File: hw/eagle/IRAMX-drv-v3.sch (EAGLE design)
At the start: 59 parts, among them IC1 IRAMTOP, IC2 STM32F103R6T, IC3 78L05SMD, IC4 78L05SMD

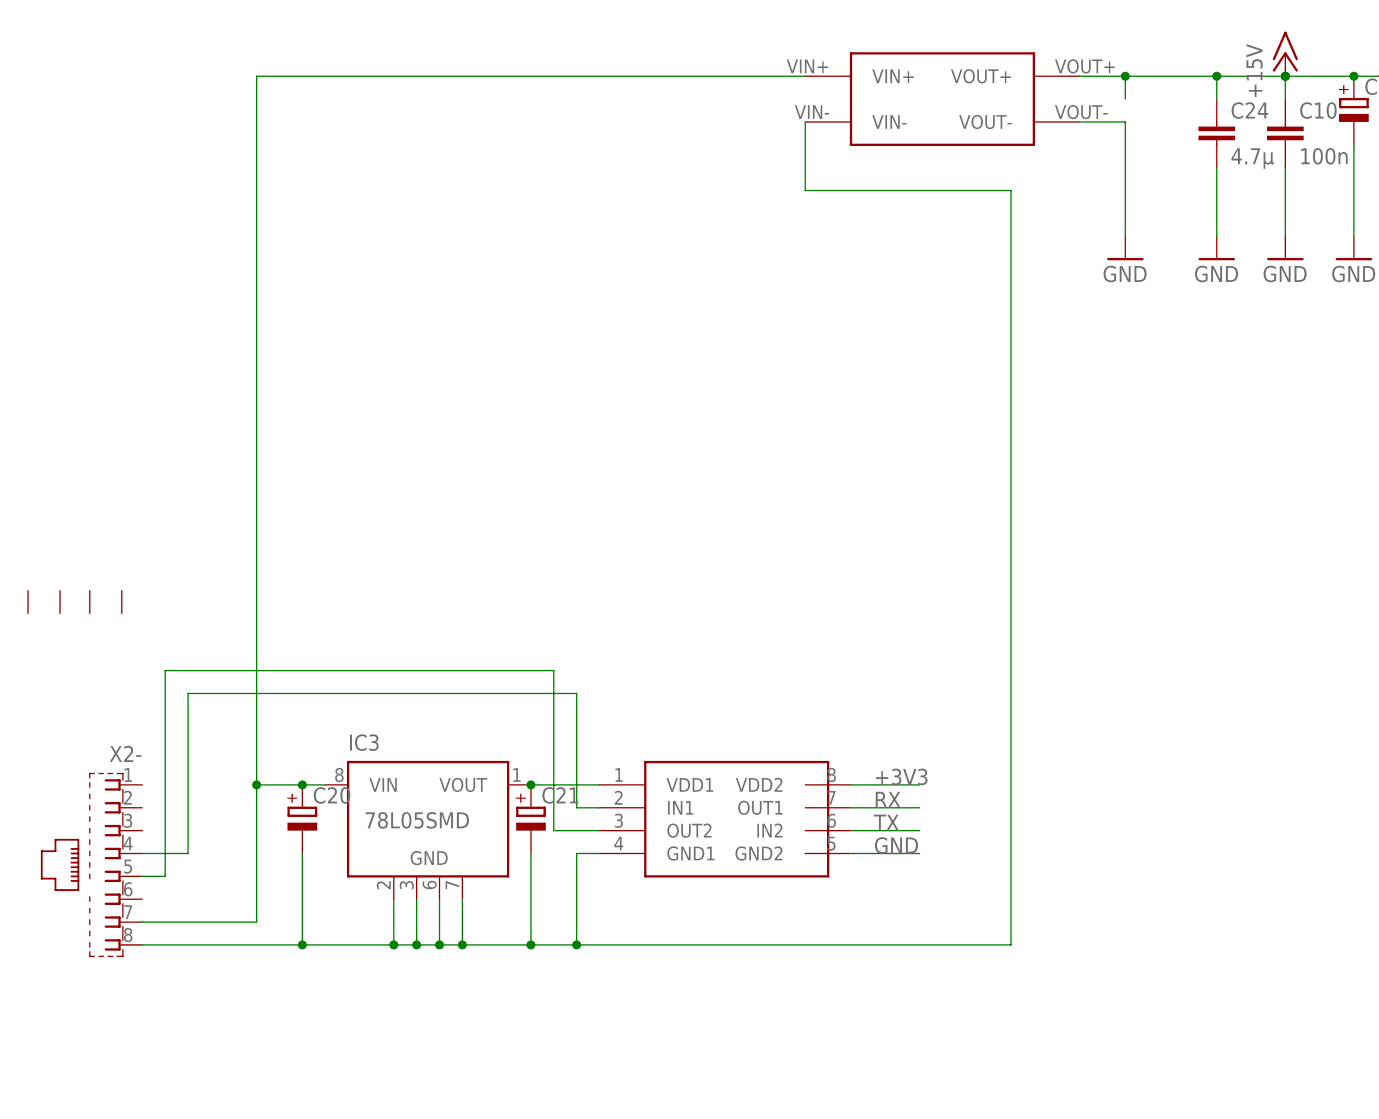
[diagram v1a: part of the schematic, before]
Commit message: iramx v3
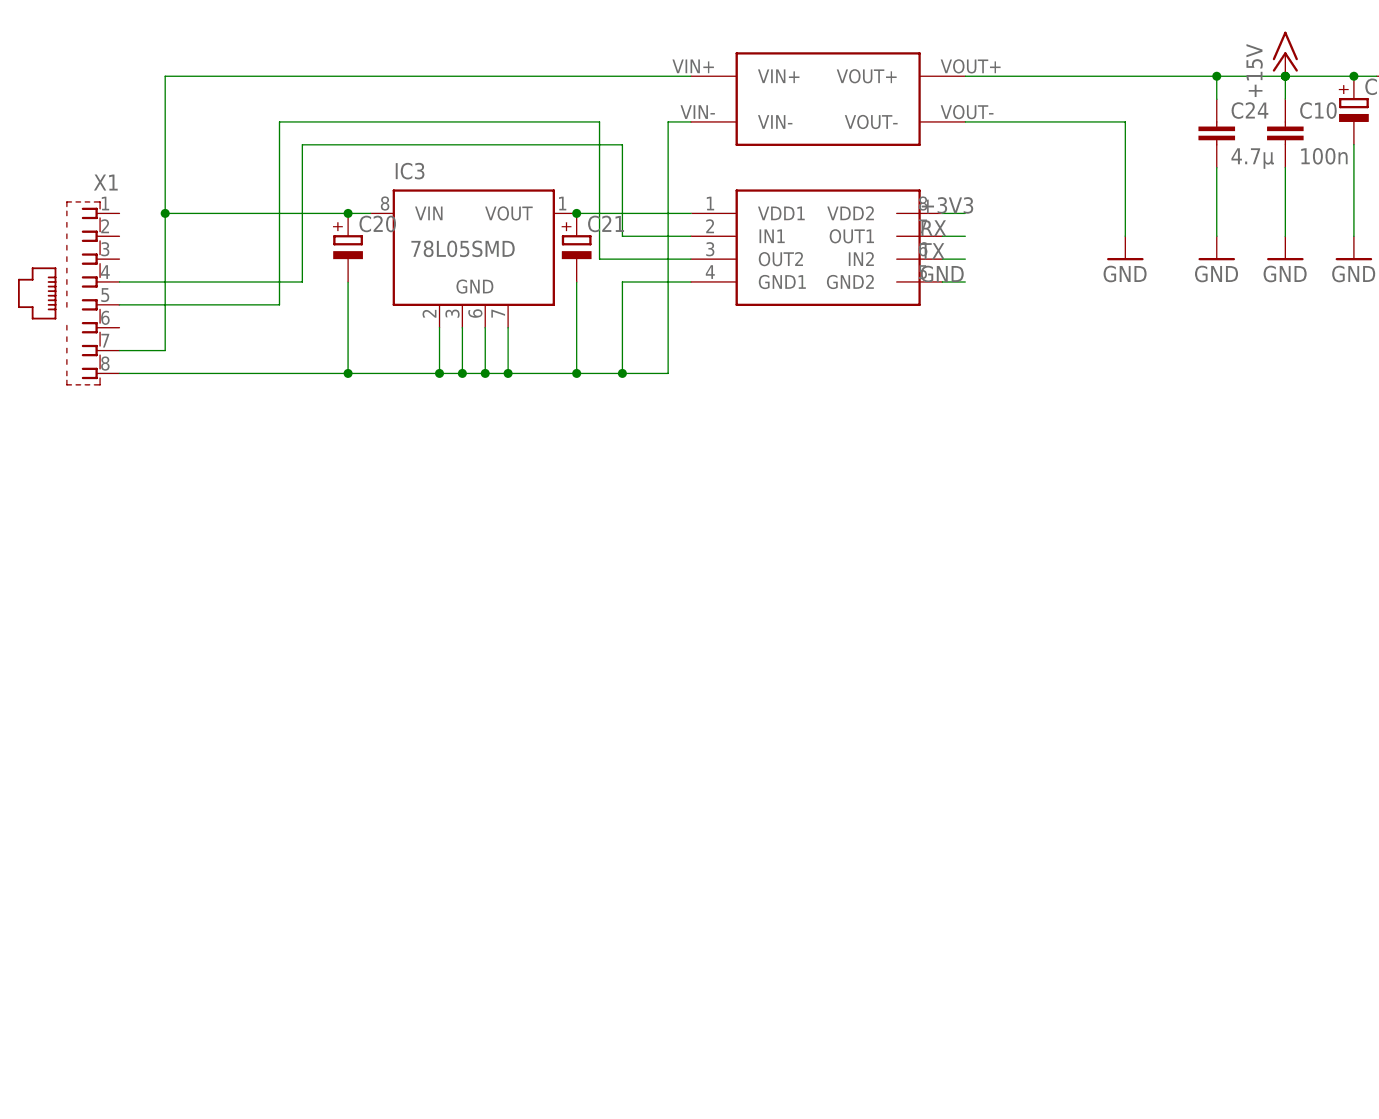
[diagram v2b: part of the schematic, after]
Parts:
- removed X2: (no value), con-appsys:RJ45
- added X1: (no value), reroolib:RJ45
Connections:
- net ISO_GND: now also X1.8; no longer X2-.8
- net N$13: now also X1.4; no longer X2-.4
- net N$14: now also X1.5; no longer X2-.5
- net N$17: now also X1.7; no longer X2-.7
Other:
- moved on the sheet: C20, C21, IC3
